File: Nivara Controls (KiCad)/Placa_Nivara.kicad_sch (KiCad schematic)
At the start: 3 parts, among them U2 ESP32-S3-WROOM-1

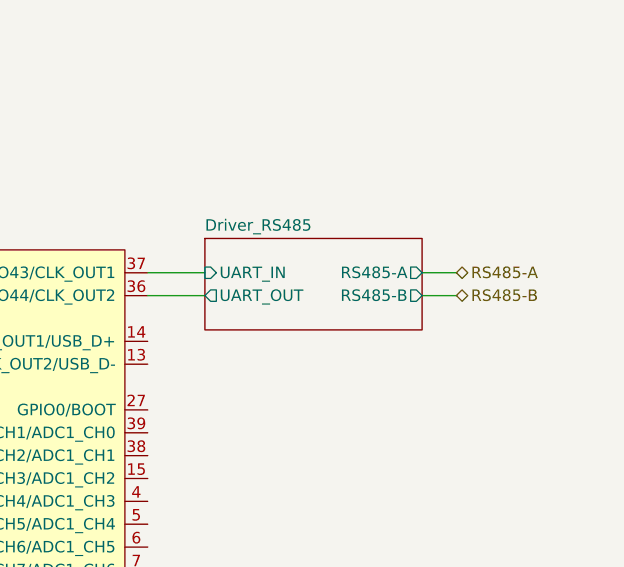
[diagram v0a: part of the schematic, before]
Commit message: TVS
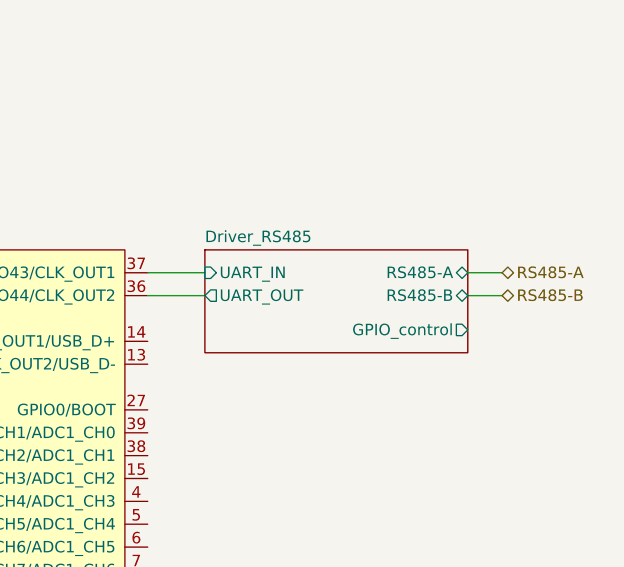
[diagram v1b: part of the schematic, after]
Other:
- sheet Driver_RS485 ports: added GPIO_control; removed none
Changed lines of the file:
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@@
+	(wire
+		(pts
+			(xy 92.71 80.01) (xy 92.71 81.28)
+		)
+		(stroke
+			(width 0)
+			(type default)
+		)
+	)
+	(wire
+		(pts
+			(xy 85.09 87.63) (xy 85.09 81.28)
+		)
+		(stroke
+			(width 0)
+			(type default)
+		)
+	)
+	(wire
+		(pts
+			(xy 154.94 156.21) (xy 154.94 158.75)
+		)
+		(stroke
+			(width 0)
+			(type default)
+		)
+	)
+	(wire
+		(pts
+			(xy 92.71 81.28) (xy 109.22 81.28)
+		)
+		(stroke
+			(width 0)
+			(type default)
+		)
+	)
+	(wire
+		(pts
+			(xy 200.66 80.01) (xy 207.01 80.01)
+		)
+		(stroke
+			(width 0)
+			(type default)
+		)
+	)
+	(wire
+		(pts
+			(xy 85.09 95.25) (xy 85.09 99.06)
+		)
+		(stroke
+			(width 0)
+			(type default)
+		)
+	)
 	(wire
 		(pts
@@
 	(wire
 		(pts
-			(xy 92.71 80.01) (xy 92.71 81.28)
-		)
-		(stroke
-			(width 0)
-			(type default)
-		)
-	)
-	(wire
-		(pts
-			(xy 85.09 87.63) (xy 85.09 81.28)
-		)
-		(stroke
-			(width 0)
-			(type default)
-		)
-	)
-	(wire
-		(pts
-			(xy 154.94 156.21) (xy 154.94 158.75)
-		)
-		(stroke
-			(width 0)
-			(type default)
-		)
-	)
-	(wire
-		(pts
-			(xy 92.71 81.28) (xy 109.22 81.28)
-		)
-		(stroke
-			(width 0)
-			(type default)
-		)
-	)
-	(wire
-		(pts
-			(xy 85.09 95.25) (xy 85.09 99.06)
-		)
-		(stroke
-			(width 0)
-			(type default)
-		)
-	)
-	(wire
-		(pts
-			(xy 231.14 80.01) (xy 234.95 80.01)
-		)
-		(stroke
-			(width 0)
-			(type default)
-		)
-	)
-	(wire
-		(pts
 			(xy 92.71 71.12) (xy 96.52 71.12)
 		)
@@
 	(wire
 		(pts
-			(xy 231.14 82.55) (xy 234.95 82.55)
+			(xy 236.22 82.55) (xy 240.03 82.55)
 		)
 		(stroke
@@
 	(wire
 		(pts
-			(xy 200.66 80.01) (xy 207.01 80.01)
+			(xy 236.22 80.01) (xy 240.03 80.01)
 		)
 		(stroke
@@
 	(hierarchical_label "RS485-B"
 		(shape bidirectional)
-		(at 234.95 82.55 0)
+		(at 240.03 82.55 0)
 		(effects
 			(font
@@
 	(hierarchical_label "RS485-A"
 		(shape bidirectional)
-		(at 234.95 80.01 0)
+		(at 240.03 80.01 0)
 		(effects
 			(font
@@
 	)
 	(sheet
-		(at 207.01 76.2)
-		(size 24.13 10.16)
+		(at 207.01 77.47)
+		(size 29.21 11.43)
 		(exclude_from_sim no)
 		(in_bom yes)
@@
 		)
 		(property "Sheetname" "Driver_RS485"
-			(at 207.01 75.4884 0)
+			(at 207.01 76.7584 0)
 			(effects
 				(font
@@
 		)
 		(property "Sheetfile" "Driver_RS485.kicad_sch"
-			(at 207.01 86.9446 0)
+			(at 207.01 89.4846 0)
 			(effects
 				(font
@@
 			)
 		)
-		(pin "RS485-A" output
-			(at 231.14 80.01 0)
+		(pin "GPIO_control" output
+			(at 236.22 86.36 0)
 			(effects
 				(font
@@
 			)
 		)
-		(pin "RS485-B" output
-			(at 231.14 82.55 0)
-			(effects
-				(font
+		(pin "RS485-A" bidirectional
+			(at 236.22 80.01 0)
+			(effects
+				(font
+					(size 1.27 1.27)
+				)
+				(justify right)
+			)
+		)
+		(pin "RS485-B" bidirectional
+			(at 236.22 82.55 0)
+			(effects
+				(font
